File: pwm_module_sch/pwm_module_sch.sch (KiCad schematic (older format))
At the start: 15 parts

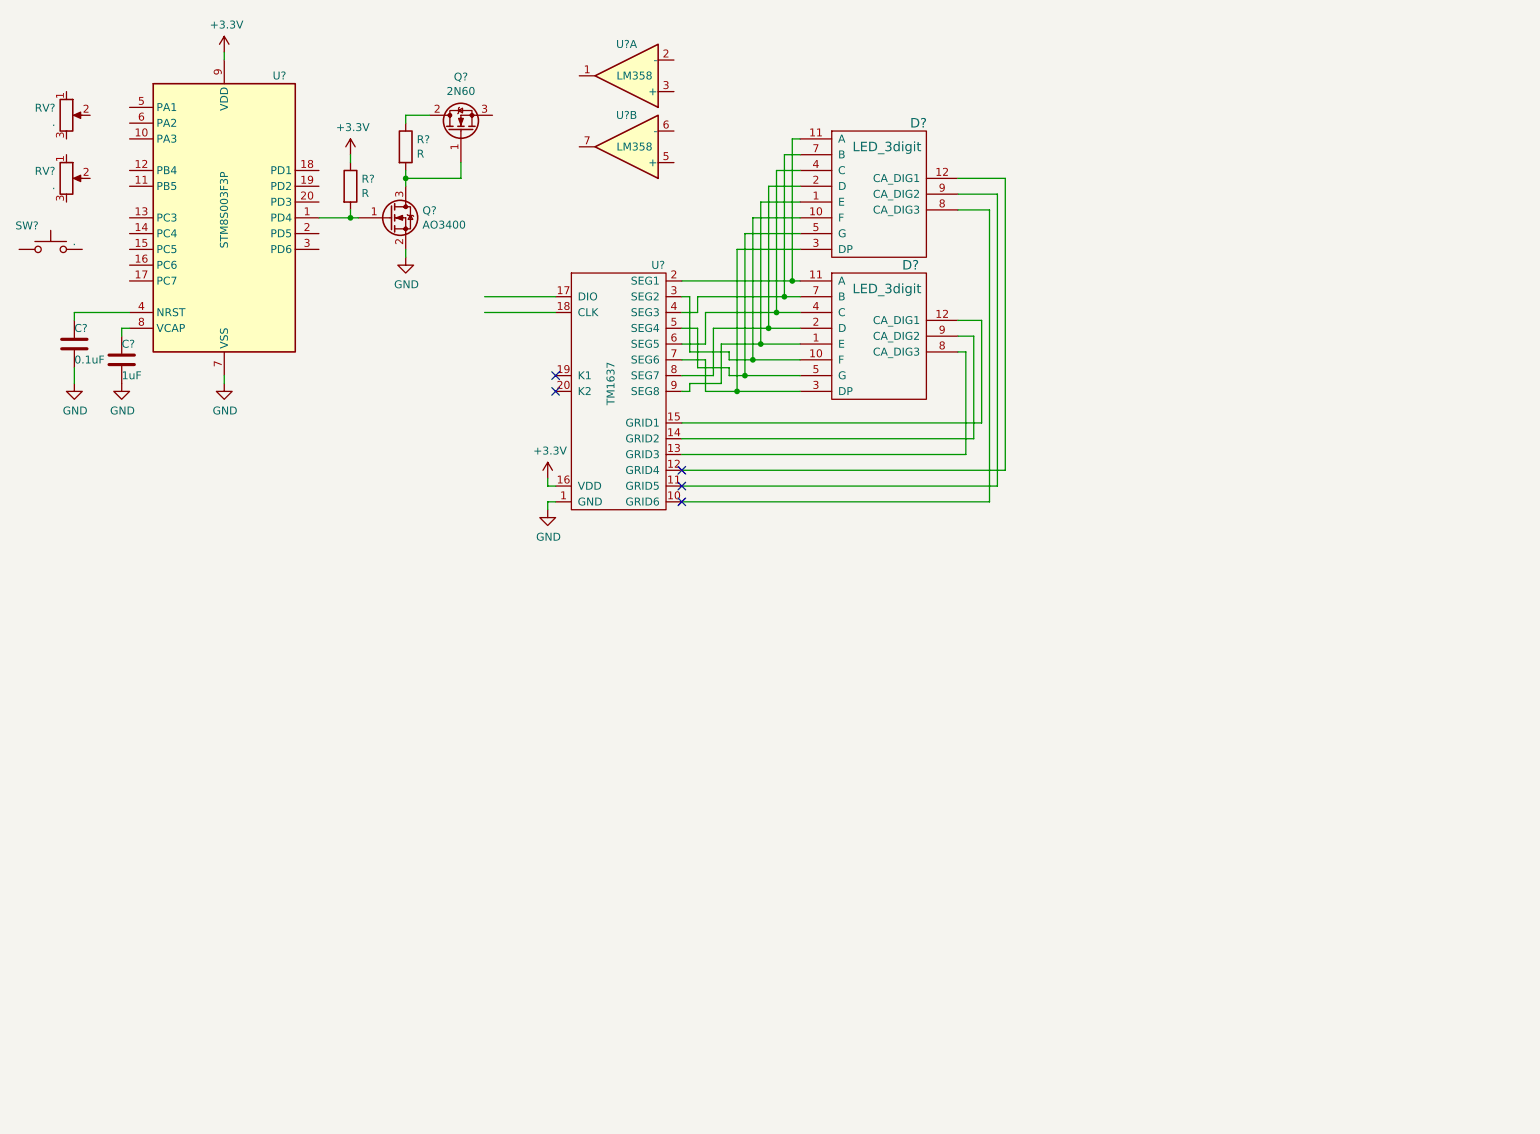
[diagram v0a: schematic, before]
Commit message: schermatic
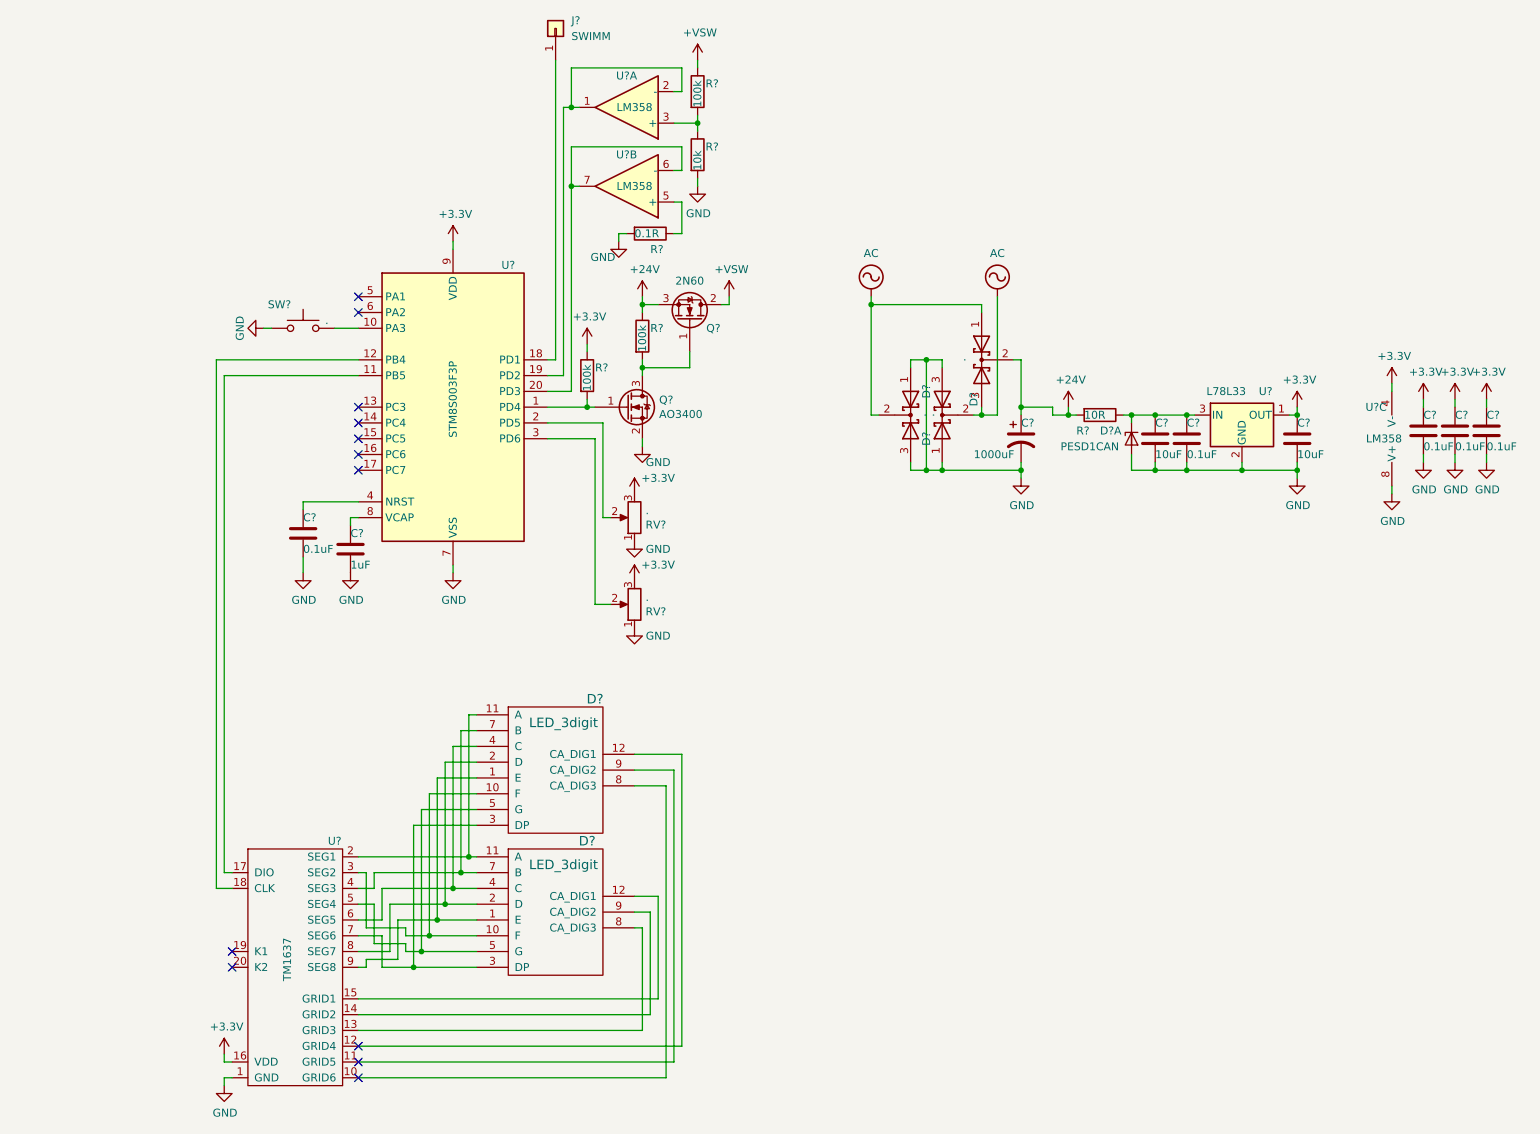
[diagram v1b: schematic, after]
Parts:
- added C? (x2): 10uF, symbol Device:C
- added C? (x4): 0.1uF, symbol Device:C
- added C?: 1000uF, symbol Device:C_Polarized_US
- added D? (x3): ., symbol Device:D_Schottky_Dual_CommonCathode_AKA
- added D?: PESD1CAN, Package_TO_SOT_SMD:SOT-886, symbol Power_Protection:PESD3V3L4UF
- added J?: SWIMM, symbol Connector_Generic:Conn_01x01
- added R?: 0.1R, symbol Device:R
- added R?: 100k, symbol Device:R
- added R?: 10k, symbol Device:R
- added R?: 10R, symbol Device:R
- added U?: L78L33, Package_TO_SOT_SMD:SOT-89-3, symbol Regulator_Linear:L78L33_SOT89
- added U?: LM358, symbol Amplifier_Operational:LM358
- R? (x2): value R -> 100k
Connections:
- net +3V3: now also RV?.3, RV?.3, C?.1, C?.1, C?.1, C?.1, U?.1 (OUT), U?.4 (V-)
- net GND: now also RV?.1, RV?.1, SW?.1, C?.2, C?.2, C?.2, C?.2, C?.2, C?.2, C?.2, D?.1 (A), D?.1 (A), D?.2 (A), D?.3 (A), D?.3 (A), D?.5 (A), R?.2, R?.2, U?.2 (GND), U?.8 (V+)
- net at U?.17 (DIO): now also U?.11 (PB5)
- net at U?.18 (CLK): now also U?.12 (PB4)
- net at U?.10 (PA3): now also SW?.2
- net at U?.18 (PD1): now also J?.1 (Pin_1)
- net at U?.19 (PD2): now also U?.1, U?.2 (-)
- net at U?.2 (PD5): now also RV?.2
- net at U?.20 (PD3): now also U?.6 (-), U?.7
- net at U?.3 (PD6): now also RV?.2
- net +24V: now reaches R?.1
- net +24V: now also Q?.3 (S), C?.1, D?.2 (K), R?.2; no longer Q?.2 (D)
- net at U?.3 (+): now also R?.1, R?.2
- net at U?.5 (+): now also R?.1
- new net: C?.1, C?.1, D?.1 (K1), R?.1, U?.3 (IN)
- new net +VSW: Q?.2 (D), R?.1
- new net AC: D?.1 (A), D?.2 (K), D?.2 (K), D?.3 (A)
- no-connect marks 5 -> 12
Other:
- moved on the sheet: C?, D?, Q?, R?, RV?, SW?, U?, U?A, U?B
